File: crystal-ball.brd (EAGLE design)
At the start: 68.6 x 53.3 mm, 9 parts

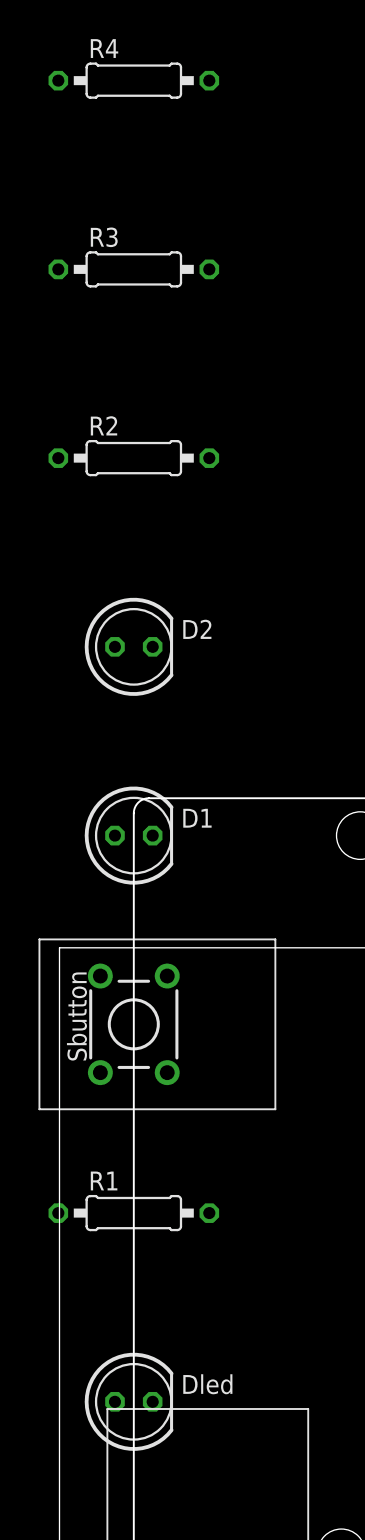
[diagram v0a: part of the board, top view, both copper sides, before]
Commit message: Added code and brd
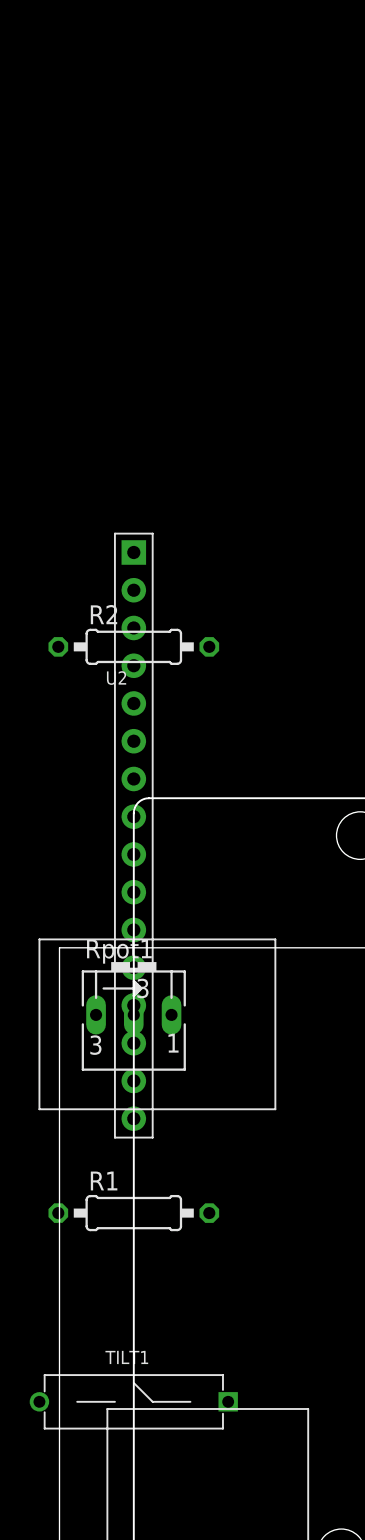
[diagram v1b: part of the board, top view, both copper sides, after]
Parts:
- removed D1, D2, Dled: (no value), AUTODESK_CIRCUITS_BREADBOARD:LED5MM
- removed R3, R4: 1k‎Ω, AUTODESK_CIRCUITS_BREADBOARD:0207/10
- removed Sbutton: (no value), AUTODESK_CIRCUITS_BREADBOARD:TL1105
- added Rpot1: 250k‎Ω, AUTODESK_CIRCUITS_BREADBOARD:B25V
- added TILT1: (no value), AUTODESK_CIRCUITS_BREADBOARD:SW2-12.7-12.0X3.6X3.6MM
- added U2: (no value), AUTODESK_CIRCUITS_BREADBOARD:1X16P-2.54-2.54-11.6-3.0-BLACK-MALE
- R1: value 1k‎Ω -> 10k‎Ω
- R2: value 1k‎Ω -> 220‎Ω
- moved R2 12.7 mm to (5.00, 73.6)
- renumbered Uboard to U1
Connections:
- new net N$12: U2.7
- new net N$13: U2.8
- new net N$14: U1.2, U2.14
- new net N$15: Rpot1.S, U2.3
- net N$1: now also TILT1.2, U1.6; no longer R2.1, R3.1, R4.1, U1.GND..
- net N$10: now also U1.3, U2.13; no longer Sbutton.2
- net N$11: now also R2.1, U2.15; no longer Sbutton.1
- net N$2: now also R2.2, Rpot1.A, TILT1.1, U2.2; no longer Sbutton.3
- net N$3: now also U1.12, U2.4; no longer Dled.K, R4.2
- net N$4: now also R1.2, Rpot1.E, U1.GND.., U2.1, U2.16, U2.5; no longer Dled.A, U1.3
- net N$5: now also U1.11, U2.6; no longer D2.K, R1.2
- net N$6: now also U2.9; no longer D2.A, U1.5
- net N$7: now also U2.10; no longer D1.K, R3.2
- net N$8: now also U1.5, U2.11; no longer D1.A, U1.4
- net N$9: now also U1.4, U2.12; no longer R2.2, Sbutton.4, U1.2
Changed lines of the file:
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@@
 </autorouter>
 <elements>
-<element value="" name="Uboard" library="AUTODESK_CIRCUITS_BREADBOARD" package="ARDUINO_UNO" x="5" y="10.08"></element><element value="" name="Dled" library="AUTODESK_CIRCUITS_BREADBOARD" package="LED5MM" x="5" y="22.78"></element><element value="1k‎Ω" name="R1" library="AUTODESK_CIRCUITS_BREADBOARD" package="0207/10" x="5" y="35.480000000000004"></element><element value="" name="Sbutton" library="AUTODESK_CIRCUITS_BREADBOARD" package="TL1105" x="5" y="48.18"></element><element value="" name="D1" library="AUTODESK_CIRCUITS_BREADBOARD" package="LED5MM" x="5" y="60.879999999999995"></element><element value="" name="D2" library="AUTODESK_CIRCUITS_BREADBOARD" package="LED5MM" x="5" y="73.58"></element><element value="1k‎Ω" name="R2" library="AUTODESK_CIRCUITS_BREADBOARD" package="0207/10" x="5" y="86.28"></element><element value="1k‎Ω" name="R3" library="AUTODESK_CIRCUITS_BREADBOARD" package="0207/10" x="5" y="98.98"></element><element value="1k‎Ω" name="R4" library="AUTODESK_CIRCUITS_BREADBOARD" package="0207/10" x="5" y="111.68"></element></elements>
+<element value="" name="U1" library="AUTODESK_CIRCUITS_BREADBOARD" package="ARDUINO_UNO" x="5" y="10.08"></element><element value="" name="TILT1" library="AUTODESK_CIRCUITS_BREADBOARD" package="SW2-12.7-12.0X3.6X3.6MM" x="5" y="22.78"></element><element value="10k‎Ω" name="R1" library="AUTODESK_CIRCUITS_BREADBOARD" package="0207/10" x="5" y="35.480000000000004"></element><element value="250k‎Ω" name="Rpot1" library="AUTODESK_CIRCUITS_BREADBOARD" package="B25V" x="5" y="48.18"></element><element value="" name="U2" library="AUTODESK_CIRCUITS_BREADBOARD" package="1X16P-2.54-2.54-11.6-3.0-BLACK-MALE" x="5" y="60.879999999999995"></element><element value="220‎Ω" name="R2" library="AUTODESK_CIRCUITS_BREADBOARD" package="0207/10" x="5" y="73.58"></element></elements>
 <signals>
-<signal name="N$1"><contactref element="Uboard" pad="GND.."></contactref><contactref element="R2" pad="1"></contactref><wire x1="45.64" y1="12.620000000000001" x2="-0.08000000000000007" y2="86.28" width="0" layer="19" extent="1-1"></wire><contactref element="R1" pad="1"></contactref><wire x1="-0.08000000000000007" y1="86.28" x2="-0.08000000000000007" y2="35.480000000000004" width="0" layer="19" extent="1-1"></wire><contactref element="R3" pad="1"></contactref><wire x1="-0.08000000000000007" y1="35.480000000000004" x2="-0.08000000000000007" y2="98.98" width="0" layer="19" extent="1-1"></wire><contactref element="R4" pad="1"></contactref><wire x1="-0.08000000000000007" y1="98.98" x2="-0.08000000000000007" y2="111.68" width="0" layer="19" extent="1-1"></wire></signal><signal name="N$2"><contactref element="Uboard" pad="5V"></contactref><contactref element="Sbutton" pad="3"></contactref><wire x1="43.1" y1="12.620000000000001" x2="2.75" y2="44.93" width="0" layer="19" extent="1-1"></wire></signal><signal name="N$3"><contactref element="Dled" pad="K"></contactref><contactref element="R4" pad="2"></contactref><wire x1="6.27" y1="22.78" x2="10.08" y2="111.68" width="0" layer="19" extent="1-1"></wire></signal><signal name="N$4"><contactref element="Dled" pad="A"></contactref><contactref element="Uboard" pad="3"></contactref><wire x1="3.73" y1="22.78" x2="60.88" y2="60.879999999999995" width="0" layer="19" extent="1-1"></wire></signal><signal name="N$5"><contactref element="D2" pad="K"></contactref><contactref element="R1" pad="2"></contactref><wire x1="6.27" y1="73.58" x2="10.08" y2="35.480000000000004" width="0" layer="19" extent="1-1"></wire></signal><signal name="N$6"><contactref element="D2" pad="A"></contactref><contactref element="Uboard" pad="5"></contactref><wire x1="3.73" y1="73.58" x2="55.8" y2="60.879999999999995" width="0" layer="19" extent="1-1"></wire></signal><signal name="N$7"><contactref element="D1" pad="K"></contactref><contactref element="R3" pad="2"></contactref><wire x1="6.27" y1="60.879999999999995" x2="10.08" y2="98.98" width="0" layer="19" extent="1-1"></wire></signal><signal name="N$8"><contactref element="D1" pad="A"></contactref><contactref element="Uboard" pad="4"></contactref><wire x1="3.73" y1="60.879999999999995" x2="58.34" y2="60.879999999999995" width="0" layer="19" extent="1-1"></wire></signal><signal name="N$9"><contactref element="Sbutton" pad="4"></contactref><contactref element="Uboard" pad="2"></contactref><wire x1="7.25" y1="44.93" x2="63.42" y2="60.879999999999995" width="0" layer="19" extent="1-1"></wire><contactref element="R2" pad="2"></contactref><wire x1="63.42" y1="60.879999999999995" x2="10.08" y2="86.28" width="0" layer="19" extent="1-1"></wire></signal><signal name="N$10"><contactref element="Sbutton" pad="2"></contactref></signal><signal name="N$11"><contactref element="Sbutton" pad="1"></contactref></signal></signals>
+<signal name="N$1"><contactref element="U1" pad="6"></contactref><contactref element="TILT1" pad="2"></contactref><wire x1="53.26" y1="60.879999999999995" x2="-1.3499999999999996" y2="22.78" width="0" layer="19" extent="1-1"></wire><contactref element="R1" pad="1"></contactref><wire x1="-1.3499999999999996" y1="22.78" x2="-0.08000000000000007" y2="35.480000000000004" width="0" layer="19" extent="1-1"></wire></signal><signal name="N$2"><contactref element="U2" pad="2"></contactref><contactref element="Rpot1" pad="A"></contactref><wire x1="5" y1="77.39" x2="7.54" y2="48.815" width="0" layer="19" extent="1-1"></wire><contactref element="U1" pad="5V"></contactref><wire x1="7.54" y1="48.815" x2="43.1" y2="12.620000000000001" width="0" layer="19" extent="1-1"></wire><contactref element="TILT1" pad="1"></contactref><wire x1="43.1" y1="12.620000000000001" x2="11.35" y2="22.78" width="0" layer="19" extent="1-1"></wire><contactref element="R2" pad="2"></contactref><wire x1="11.35" y1="22.78" x2="10.08" y2="73.58" width="0" layer="19" extent="1-1"></wire></signal><signal name="N$3"><contactref element="U2" pad="4"></contactref><contactref element="U1" pad="12"></contactref><wire x1="5" y1="72.31" x2="36.495999999999995" y2="60.879999999999995" width="0" layer="19" extent="1-1"></wire></signal><signal name="N$4"><contactref element="U2" pad="5"></contactref><contactref element="U2" pad="16"></contactref><wire x1="5" y1="69.77" x2="5" y2="41.83" width="0" layer="19" extent="1-1"></wire><contactref element="U2" pad="1"></contactref><wire x1="5" y1="41.83" x2="5" y2="79.92999999999999" width="0" layer="19" extent="1-1"></wire><contactref element="Rpot1" pad="E"></contactref><wire x1="5" y1="79.92999999999999" x2="2.46" y2="48.815" width="0" layer="19" extent="1-1"></wire><contactref element="R1" pad="2"></contactref><wire x1="2.46" y1="48.815" x2="10.08" y2="35.480000000000004" width="0" layer="19" extent="1-1"></wire><contactref element="U1" pad="GND.."></contactref><wire x1="10.08" y1="35.480000000000004" x2="45.64" y2="12.620000000000001" width="0" layer="19" extent="1-1"></wire></signal><signal name="N$5"><contactref element="U2" pad="6"></contactref><contactref element="U1" pad="11"></contactref><wire x1="5" y1="67.22999999999999" x2="39.036" y2="60.879999999999995" width="0" layer="19" extent="1-1"></wire></signal><signal name="N$6"><contactref element="U2" pad="9"></contactref></signal><signal name="N$7"><contactref element="U2" pad="10"></contactref></signal><signal name="N$8"><contactref element="U2" pad="11"></contactref><contactref element="U1" pad="5"></contactref><wire x1="5" y1="54.529999999999994" x2="55.8" y2="60.879999999999995" width="0" layer="19" extent="1-1"></wire></signal><signal name="N$9"><contactref element="U2" pad="12"></contactref><contactref element="U1" pad="4"></contactref><wire x1="5" y1="51.989999999999995" x2="58.34" y2="60.879999999999995" width="0" layer="19" extent="1-1"></wire></signal><signal name="N$10"><contactref element="U2" pad="13"></contactref><contactref element="U1" pad="3"></contactref><wire x1="5" y1="49.449999999999996" x2="60.88" y2="60.879999999999995" width="0" layer="19" extent="1-1"></wire></signal><signal name="N$11"><contactref element="U2" pad="15"></contactref><contactref element="R2" pad="1"></contactref><wire x1="5" y1="44.36999999999999" x2="-0.08000000000000007" y2="73.58" width="0" layer="19" extent="1-1"></wire></signal><signal name="N$12"><contactref element="U2" pad="7"></contactref></signal><signal name="N$13"><contactref element="U2" pad="8"></contactref></signal><signal name="N$14"><contactref element="U2" pad="14"></contactref><contactref element="U1" pad="2"></contactref><wire x1="5" y1="46.91" x2="63.42" y2="60.879999999999995" width="0" layer="19" extent="1-1"></wire></signal><signal name="N$15"><contactref element="Rpot1" pad="S"></contactref><contactref element="U2" pad="3"></contactref><wire x1="5" y1="48.815" x2="5" y2="74.85" width="0" layer="19" extent="1-1"></wire></signal></signals>
 </board>
 </drawing>
